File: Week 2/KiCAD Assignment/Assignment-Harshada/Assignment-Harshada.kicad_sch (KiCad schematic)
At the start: 10 parts, among them J1 USB_C_Receptacle_PowerOnly_6P, J2 Conn_01x02_Pin

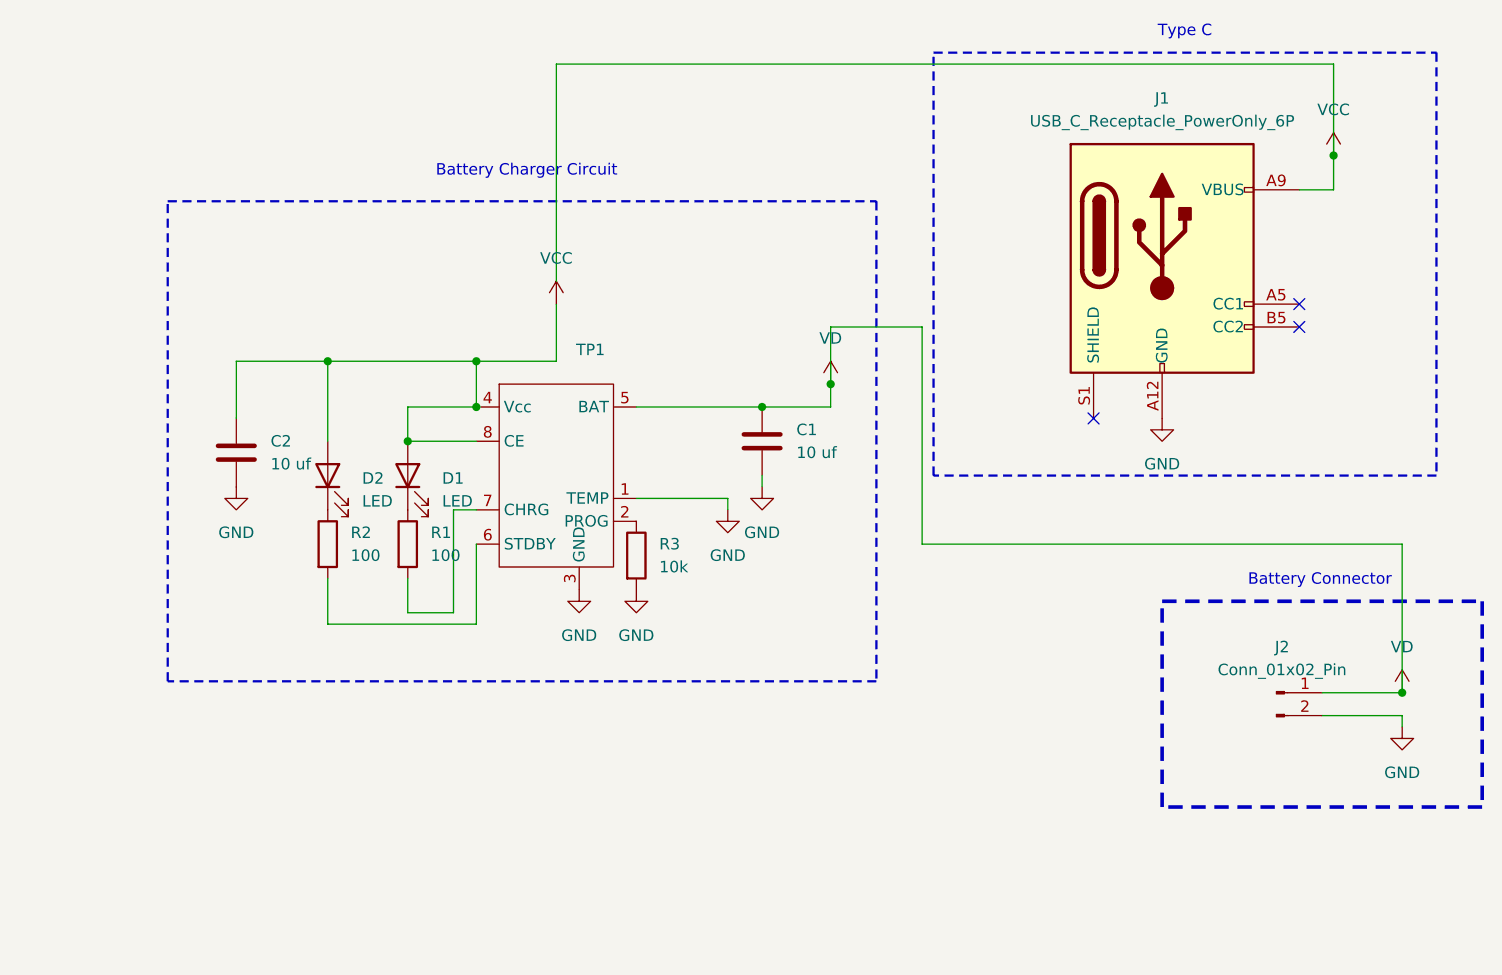
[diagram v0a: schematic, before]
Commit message: Kicad Assignment Completed
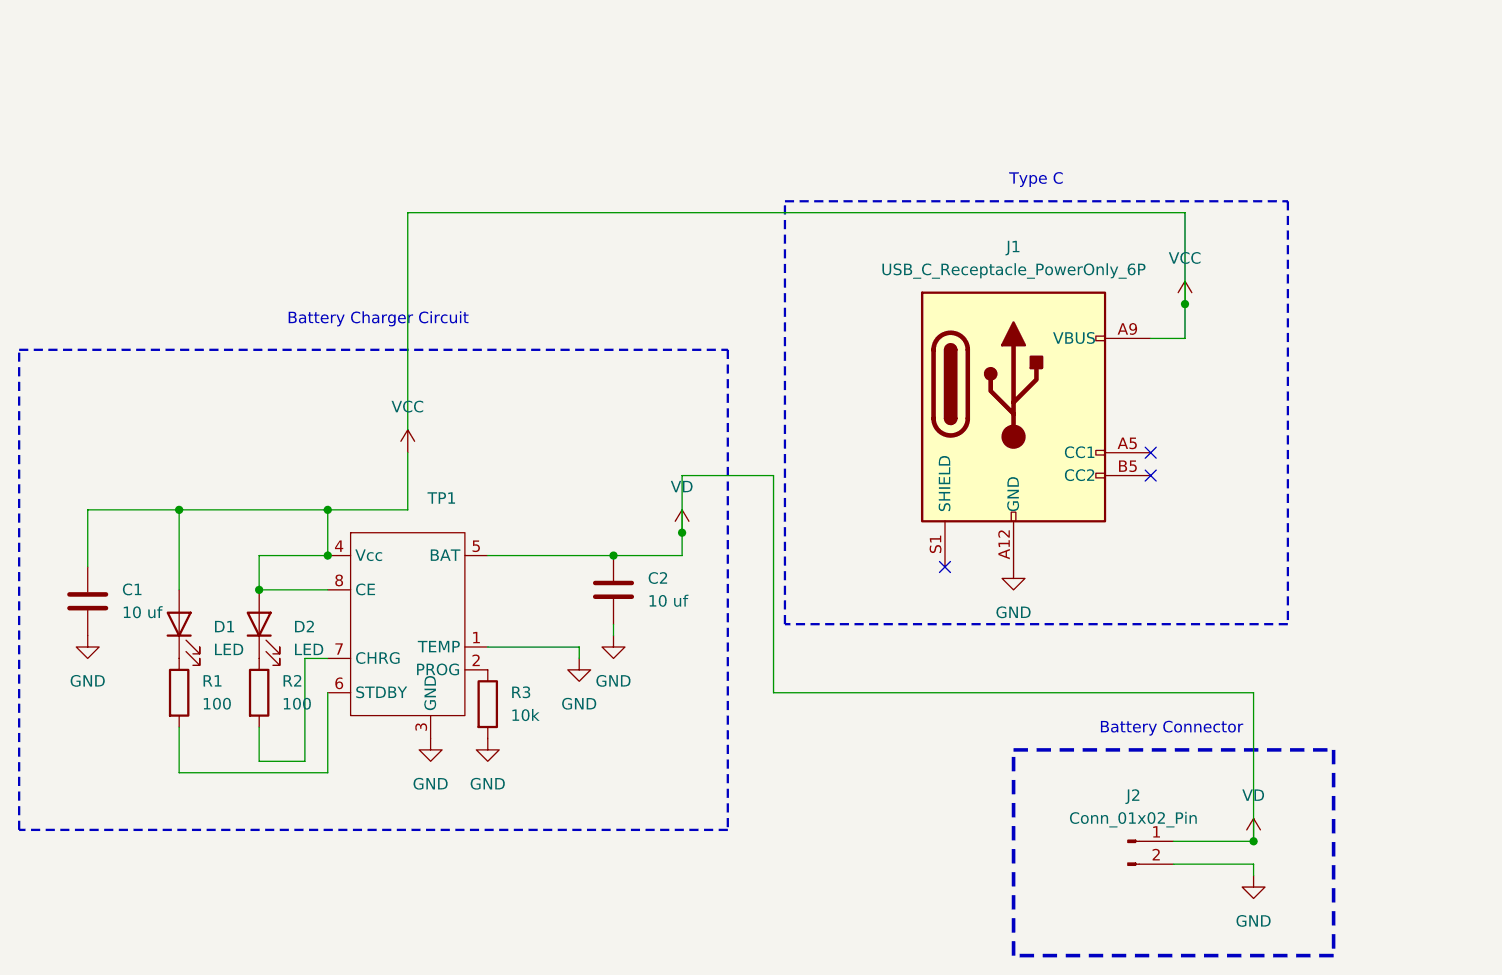
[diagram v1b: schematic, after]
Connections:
- net VCC: now also C1.1; no longer C2.1
- net VD: now also C2.1; no longer C1.1
- net at TP1.7 (CHRG): now also R2.2; no longer R1.2
- net at TP1.6 (STDBY): now also R1.2; no longer R2.2
